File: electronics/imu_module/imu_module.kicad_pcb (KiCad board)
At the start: 2 copper layers, 30 x 40 mm, 26 parts, among them J1 Conn_01x06_Male, J2 Conn_01x04, J3 Conn_01x04, SW1 SW_Push, SW2 SW_Push, SW3 SW_Push, U1 ESP32-WROOM-32U, U2 SP485, U3 ISM330DHCXTR, U4 SN74LV1T34DBVR, U5 AP2114HA-3.3TRG1

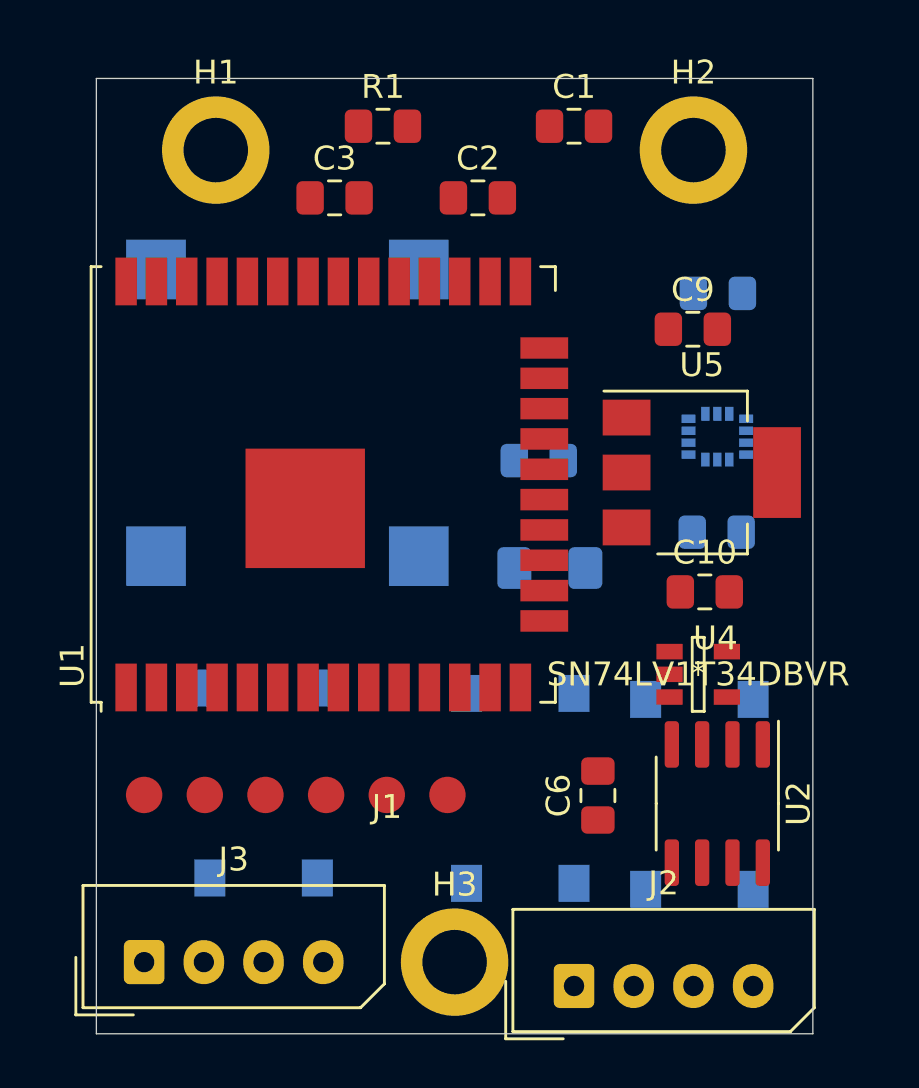
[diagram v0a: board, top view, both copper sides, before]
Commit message: hacky
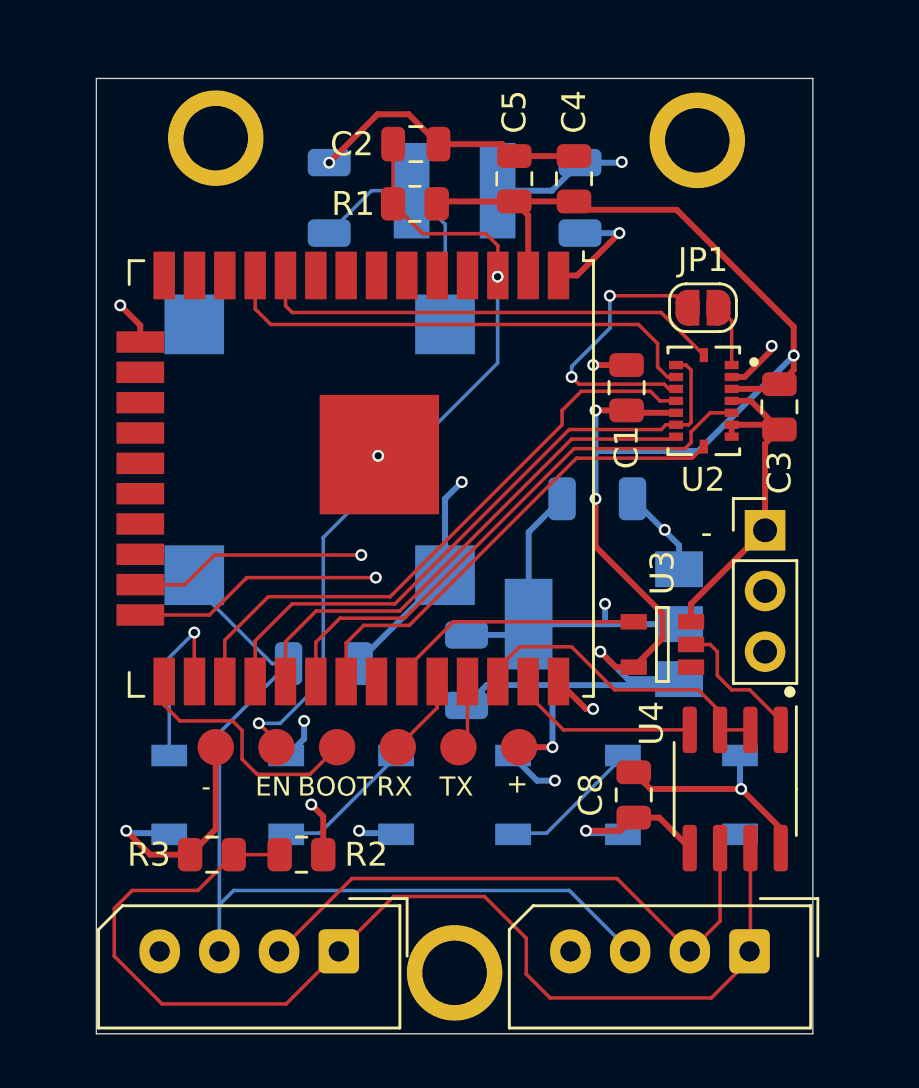
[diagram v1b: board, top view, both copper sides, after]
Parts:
- removed the C4 at (19.0, 20.5)
- removed the C5 at (18.5, 16.0)
- removed the C8 at (26.0, 9.00)
- removed SW1, SW2, SW3: SW_Push, Button_Switch_SMD:SW_SPST_B3S-1000
- removed the U3 at (26.0, 15.0)
- added C1: 100n, Capacitor_SMD:C_0805_2012Metric, F.Cu at (22.2, 12.9)
- added C3: 100n, Capacitor_SMD:C_0805_2012Metric, F.Cu at (28.6, 13.8)
- added C6: 10u/50V, Capacitor_SMD:C_1206_3216Metric, B.Cu at (9.53, 24.5)
- added C9: 22u/16v, Capacitor_SMD:C_1206_3216Metric, B.Cu at (20.2, 5.00)
- added D1: WS2812B, lib:LED_WS2812B_PLCC4_5.0x5.0mm_P3.2mm_marked, B.Cu at (5.50, 30.0)
- added D2: WS2812B, lib:LED_WS2812B_PLCC4_5.0x5.0mm_P3.2mm_marked, B.Cu at (15.0, 30.0)
- added D3: WS2812B, lib:LED_WS2812B_PLCC4_5.0x5.0mm_P3.2mm_marked, B.Cu at (24.5, 30.0)
- added G***: LOGO, bitbots:bitbots_logo, B.Cu at (21.8, 12.3)
- added J2: Conn_01x03_Male, Connector_PinHeader_2.54mm:PinHeader_1x03_P2.54mm_Vertical, F.Cu at (28.0, 18.9)
- added JP1: SolderJumper_2_Open, Jumper:SolderJumper-2_P1.3mm_Open_RoundedPad1.0x1.5mm, F.Cu at (25.4, 9.60)
- added L1: 22uH, lib:VLS5045EX330M, B.Cu at (15.0, 4.70)
- added R2: 4K7, Resistor_SMD:R_0805_2012Metric, F.Cu at (8.59, 32.5)
- added R3: 4K7, Resistor_SMD:R_0805_2012Metric, F.Cu at (4.84, 32.5)
- added U2: BMI088, lib:PQFN50P450X300X100-16N, F.Cu at (25.4, 13.5)
- C10: renamed from C9; footprint Capacitor_SMD:C_0805_2012Metric_Pad1.15x1.40mm_HandSolder -> Capacitor_SMD:C_1206_3216Metric; moved to B.Cu
- C11: renamed from C10; footprint Capacitor_SMD:C_0805_2012Metric_Pad1.15x1.40mm_HandSolder -> Capacitor_SMD:C_1206_3216Metric; moved to B.Cu
- C2: renamed from C1; footprint Capacitor_SMD:C_0805_2012Metric_Pad1.15x1.40mm_HandSolder -> Capacitor_SMD:C_0805_2012Metric
- C4: renamed from C2; footprint Capacitor_SMD:C_0805_2012Metric_Pad1.15x1.40mm_HandSolder -> Capacitor_SMD:C_0805_2012Metric
- C5: renamed from C3; footprint Capacitor_SMD:C_0805_2012Metric_Pad1.15x1.40mm_HandSolder -> Capacitor_SMD:C_0805_2012Metric
- C7: value 100n -> 22u/16v; footprint Capacitor_SMD:C_0805_2012Metric_Pad1.15x1.40mm_HandSolder -> Capacitor_SMD:C_1206_3216Metric
- C8: renamed from C6; footprint Capacitor_SMD:C_0805_2012Metric_Pad1.15x1.40mm_HandSolder -> Capacitor_SMD:C_0805_2012Metric
- PS1: value VXO7805-500-M -> PXO7805-500-M-TR; footprint bitbots:VXO7805-500-M -> lib:CONV_PXO7805-500-M-TR
- R1: footprint Resistor_SMD:R_0805_2012Metric_Pad1.15x1.40mm_HandSolder -> Resistor_SMD:R_0805_2012Metric
- U5: moved to B.Cu
- moved C7 21.4 mm to (9.75, 5.00), turned to 90 degrees
- moved J1 15.8 mm to (17.7, 28.0), turned to 180 degrees
- moved C11 10.5 mm to (15.5, 24.8), turned to 90 degrees
- moved J4 8.16 mm to (10.2, 36.5), turned to 180 degrees
- moved C10 8.15 mm to (21.0, 17.6), turned to 180 degrees
- moved C5 7.57 mm to (17.5, 4.20), turned to 90 degrees
- moved U5 7.56 mm to (21.2, 22.9), turned to 180 degrees
- moved J3 7.49 mm to (27.4, 36.5), turned to 180 degrees
- moved C2 6.67 mm to (13.4, 2.75)
- moved C4 4.10 mm to (20.0, 4.20), turned to 90 degrees
- moved R1 3.51 mm to (13.3, 5.25), turned to 180 degrees
- moved PS1 2.06 mm to (9.35, 15.6)
- moved U3 1.95 mm to (23.7, 23.7), turned to 180 degrees
- moved U1 1.61 mm to (11.1, 16.8), turned to -90 degrees
- moved C8 1.50 mm to (22.5, 30.0), turned to -90 degrees
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- renumbered J2 to J3, J3 to J4, U4 to U3, U2 to U4
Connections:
- C7 pad 1: +3V3 -> Net-(PS1-+VO)
- J3 pad 1: GND -> DATA-
- J3 pad 2: +1V2 -> DATA+
- J3 pad 3: DATA+ -> VBUS
- J3 pad 4: DATA- -> GND
- J4 pad 1: GND -> DATA-
- J4 pad 2: +1V2 -> DATA+
- J4 pad 3: DATA+ -> VBUS
- J4 pad 4: DATA- -> GND
- PS1 pad 1: +1V2 -> VBUS
- PS1 pad 2: GND -> (no net)
- PS1 pad 3: +5V -> Net-(PS1-+VO)
- PS1 pad 4: Net-(PS1-Pad4) -> GND
- U1 pad 10: Net-(U1-Pad10) -> int1_accel
- U1 pad 11: Net-(U1-Pad11) -> SPI_CS_ACCEL
- U1 pad 12: Net-(U1-Pad12) -> unconnected-(U1-IO27-Pad12)
- U1 pad 13: INT_ACC -> unconnected-(U1-IO14-Pad13)
- U1 pad 14: Net-(U1-Pad14) -> unconnected-(U1-IO12-Pad14)
- U1 pad 16: INT_GYR -> unconnected-(U1-IO13-Pad16)
- U1 pad 17: Net-(U1-Pad17) -> unconnected-(U1-SHD/SD2-Pad17)
- U1 pad 18: Net-(U1-Pad18) -> unconnected-(U1-SWP/SD3-Pad18)
- U1 pad 19: Net-(U1-Pad19) -> unconnected-(U1-SCS/CMD-Pad19)
- U1 pad 20: Net-(U1-Pad20) -> unconnected-(U1-SCK/CLK-Pad20)
- U1 pad 21: Net-(U1-Pad21) -> unconnected-(U1-SDO/SD0-Pad21)
- U1 pad 22: Net-(U1-Pad22) -> unconnected-(U1-SDI/SD1-Pad22)
- U1 pad 23: TX_EN -> SW2
- U1 pad 24: Net-(U1-Pad24) -> SW1
- U1 pad 26: Net-(U1-Pad26) -> LED
- U1 pad 27: U2_RX -> int3_gyro
- U1 pad 28: U2_TX -> SPI1_MISO
- U1 pad 29: SPI_CS -> SPI1_MOSI
- U1 pad 30: SPI1_SCK -> SPI_CS_GYRO
- U1 pad 31: SPI1_MISO -> SPI1_SCK
- U1 pad 32: Net-(U1-Pad32) -> unconnected-(U1-NC-Pad32)
- U1 pad 33: Net-(U1-Pad33) -> U2_RX
- U1 pad 36: Net-(U1-Pad36) -> TX_EN
- U1 pad 37: SPI1_MOSI -> U2_TX
- U1 pad 4: Net-(U1-Pad4) -> unconnected-(U1-SENSOR_VP-Pad4)
- U1 pad 5: Net-(U1-Pad5) -> unconnected-(U1-SENSOR_VN-Pad5)
- U1 pad 6: Net-(U1-Pad6) -> unconnected-(U1-IO34-Pad6)
- U1 pad 7: Net-(U1-Pad7) -> unconnected-(U1-IO35-Pad7)
- U1 pad 8: Net-(U1-Pad8) -> unconnected-(U1-IO32-Pad8)
- U1 pad 9: Net-(U1-Pad9) -> unconnected-(U1-IO33-Pad9)
- U3 pad 1: Net-(U4-Pad1) -> unconnected-(U3-NC-Pad1)
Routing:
- net GND: track 0.00 -> 82.4 mm, vias 0 -> 12
- net +3V3: track 0.00 -> 69.7 mm, vias 0 -> 5
- net DATA-: track 0.00 -> 47.1 mm
- net VBUS: track 0.00 -> 37.0 mm
- net en: track 0.00 -> 33.5 mm, vias 0 -> 2
- net SW1: track 0.00 -> 28.3 mm, vias 0 -> 1
- net SW2: track 0.00 -> 27.3 mm, vias 0 -> 1
- net SPI1_MISO: track 0.00 -> 26.6 mm
- net int3_gyro: track 0.00 -> 25.5 mm
- net +5V: track 0.00 -> 25.1 mm, vias 0 -> 6
- net DATA+: track 0.00 -> 24.6 mm
- net SPI_CS_GYRO: track 0.00 -> 23.3 mm
- net SPI1_MOSI: track 0.00 -> 21.6 mm
- net SPI_CS_ACCEL: track 0.00 -> 20.8 mm
- net SPI1_SCK: track 0.00 -> 20.0 mm
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- added copper zone on In2.Cu, net +5V
- added copper zone on In1.Cu, net GND
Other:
- copper layers 2 -> 4
- net class Default removed
- board text added: "+"
- board text added: "-"
- board text added: "BOOT"
- board text added: "EN"
- board text added: "IMU v2.0"
- board text added: "RX"
- board text added: "TX"
- board text added: "jasper@bit-bots.de"
